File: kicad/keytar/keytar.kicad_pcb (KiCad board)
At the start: 2 copper layers, 70 x 82.5 mm, 32 parts, among them J1 , J2 USB_B, J3 AudioJack2, J4 Conn_01x04, J5 USB_A, J6 Mini-DIN-6-Shielded, J7 Conn_01x04, Q1 BSS138, Q2 BSS138, U1 Pico, U2 MCP73831-2-OT

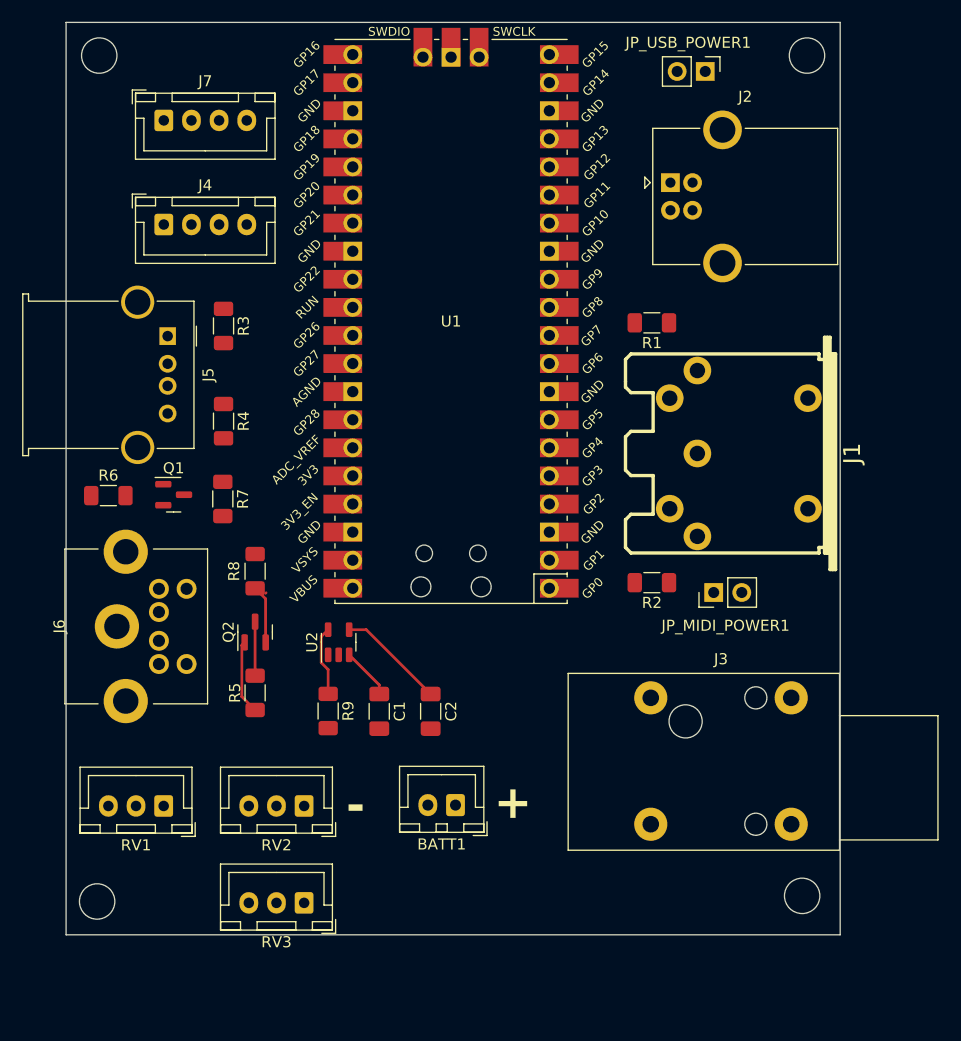
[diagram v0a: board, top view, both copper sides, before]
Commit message: route board
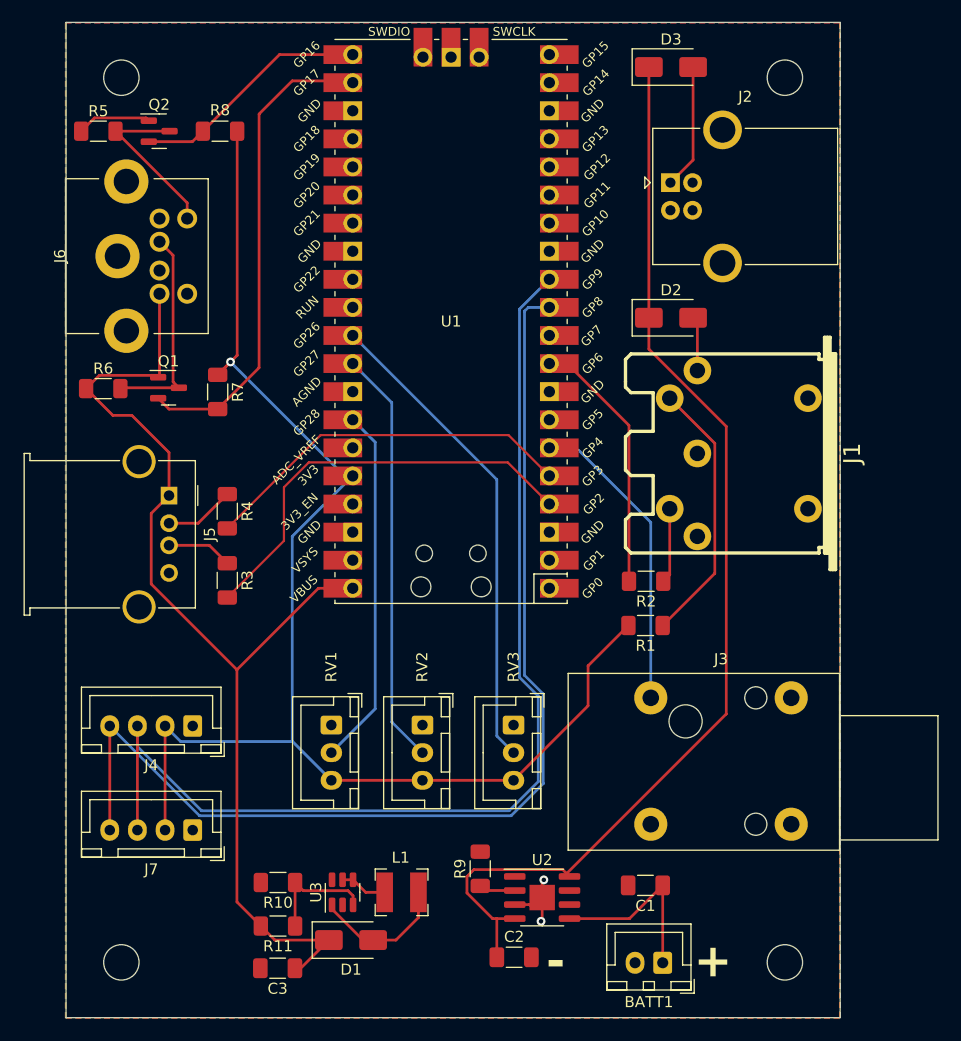
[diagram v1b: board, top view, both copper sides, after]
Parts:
- removed JP_MIDI_POWER1: MIDI Power, Connector_PinHeader_2.54mm:PinHeader_1x02_P2.54mm_Vertical
- removed JP_USB_POWER1: USB Power, Connector_PinHeader_2.54mm:PinHeader_1x02_P2.54mm_Vertical
- added C3: 22u, Capacitor_SMD:C_1206_3216Metric_Pad1.33x1.80mm_HandSolder, F.Cu at (139.1, 140.5)
- added D1: D_Schottky, Diode_SMD:D_SMA, F.Cu at (145.8, 138.0)
- added D2: D_Schottky, Diode_SMD:D_SMA, F.Cu at (174.7, 81.7)
- added D3: D_Schottky, Diode_SMD:D_SMA, F.Cu at (174.7, 59.0)
- added L1: 22u, Inductor_SMD:L_Bourns-SRN4018, F.Cu at (150.3, 133.7)
- added R10: 1k, Resistor_SMD:R_1206_3216Metric_Pad1.30x1.75mm_HandSolder, F.Cu at (139.2, 132.8)
- added R11: 7k5, Resistor_SMD:R_1206_3216Metric_Pad1.30x1.75mm_HandSolder, F.Cu at (139.2, 136.7)
- added U3: MT3608, Package_TO_SOT_SMD:SOT-23-6, F.Cu at (145.0, 133.7)
- C1: value 4u7 -> 22u
- C2: value 4u7 -> 10u
- U2: value MCP73831-2-OT -> ~; footprint Package_TO_SOT_SMD:SOT-23-5 -> Package_SO:HSOP-8-1EP_3.9x4.9mm_P1.27mm_EP2.3x2.3mm
- moved J7 64.2 mm to (131.5, 128.0), turned to 180 degrees
- moved R5 52.7 mm to (122.9, 64.8), turned to 0 degrees
- moved Q2 46.1 mm to (128.4, 64.8), turned to 0 degrees
- moved J4 45.4 mm to (131.5, 118.6), turned to 180 degrees
- moved R8 39.9 mm to (133.9, 64.8), turned to 180 degrees
- moved J6 33.5 mm to (120.0, 76.1)
- moved U2 29.5 mm to (163.1, 134.1), turned to 0 degrees
- moved C1 28.8 mm to (172.4, 133.0), turned to 180 degrees
- moved R1 27.4 mm to (172.4, 109.5)
- moved RV3 24.8 mm to (160.5, 118.5), turned to -90 degrees
- moved BATT1 23.5 mm to (174.0, 140.0)
- moved C2 23.5 mm to (160.5, 139.5), turned to 0 degrees
- moved R3 23.0 mm to (134.6, 105.5)
- moved R9 19.8 mm to (157.5, 131.5), turned to 90 degrees
- moved RV1 16.8 mm to (144.0, 118.5), turned to -90 degrees
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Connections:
- BATT1 pad 1: Net-(BATT1-Pin_1) -> +BATT
- C1 pad 1: Net-(BATT1-Pin_1) -> +BATT
- C2 pad 1: +5V -> VBUS
- J3 pad S: Net-(U1-GPIO22) -> GND
- J3 pad T: GND -> PEDAL
- RV1 pad 1: Net-(U1-AGND) -> GND
- RV1 pad 3: Net-(U1-ADC_VREF) -> +3V3
- RV2 pad 1: Net-(U1-AGND) -> GND
- RV2 pad 3: Net-(U1-ADC_VREF) -> +3V3
- RV3 pad 1: Net-(U1-AGND) -> GND
- RV3 pad 3: Net-(U1-ADC_VREF) -> +3V3
- U1 pad 29: Net-(U1-GPIO22) -> unconnected-(U1-GPIO22-Pad29)
- U1 pad 33: Net-(U1-AGND) -> unconnected-(U1-AGND-Pad33)
- U1 pad 35: Net-(U1-ADC_VREF) -> unconnected-(U1-ADC_VREF-Pad35)
- U1 pad 6: unconnected-(U1-GPIO4-Pad6) -> PEDAL
- U2 pad 1: BAT STATUS -> GND
- U2 pad 2: GND -> Net-(U2-PROG)
- U2 pad 3: Net-(BATT1-Pin_1) -> GND
- U2 pad 4: +5V -> VBUS
- U2 pad 5: Net-(U2-PROG) -> +BATT
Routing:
- net +3V3: track 0.00 -> 127.3 mm, vias 0 -> 1
- net VBUS: track 0.00 -> 102.2 mm
- net Net-(J4-Pin_4): track 0.00 -> 99.0 mm
- net Net-(J4-Pin_3): track 0.00 -> 98.3 mm
- net +5V: track 16.5 -> 102.3 mm
- net Net-(U1-GPIO26_ADC0): track 0.00 -> 43.7 mm
- net PS/2 DATA: track 0.00 -> 43.6 mm
- net USB D+: track 0.00 -> 38.6 mm
- net Net-(U1-GPIO27_ADC1): track 0.00 -> 37.8 mm
- net USB D-: track 0.00 -> 34.1 mm
- net Net-(U1-GPIO28_ADC2): track 0.00 -> 32.6 mm
- net PEDAL: track 0.00 -> 27.8 mm
- net Net-(J1-Pad4): track 0.00 -> 24.2 mm
- net MIDI TX: track 0.00 -> 22.0 mm
- net Net-(Q1-D): track 0.00 -> 19.1 mm
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- added copper zone on B.Cu, net GND
- added copper zone on F.Cu, net GND
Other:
- board size 70 x 82.5 mm -> 70 x 90 mm

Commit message: improve pcb
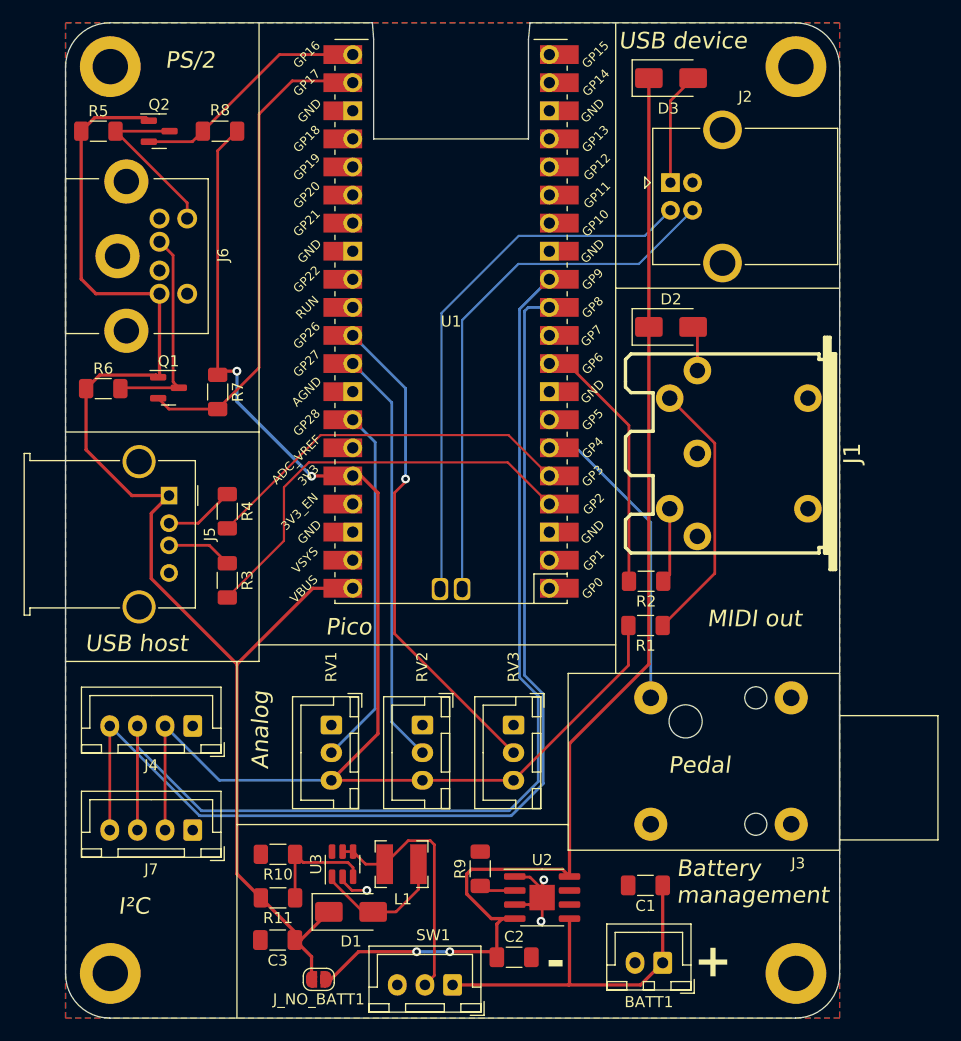
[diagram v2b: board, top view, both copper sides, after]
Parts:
- added J_NO_BATT1: Jumper_2_Open, Jumper:SolderJumper-2_P1.3mm_Open_RoundedPad1.0x1.5mm, F.Cu at (142.9, 141.5)
- added SW1: SW_DPST_x2, Connector_JST:JST_XH_B3B-XH-A_1x03_P2.50mm_Vertical, F.Cu at (155.0, 142.0)
- REF** (x4): value MountingHole_3.2mm_M3 -> MountingHole_3.2mm_M3_ISO14580_Pad; footprint MountingHole:MountingHole_3.2mm_M3 -> MountingHole:MountingHole_3.2mm_M3_ISO14580_Pad
- U1: footprint MCU_RaspberryPi_and_Boards:RPi_Pico_SMD_TH -> keyar-parts:RPi_Pico_debug_hole_USB_SMD_TH
- moved C3 2.55 mm to (139.1, 138.0)
- moved D1 2.55 mm to (145.8, 135.4)
- moved L1 2.55 mm to (150.3, 131.1)
- moved R10 2.55 mm to (139.2, 130.2)
- moved R11 2.55 mm to (139.2, 134.2)
- moved U3 2.55 mm to (145.0, 131.1)
- moved REF** 1.41 mm to (124.0, 141.0)
- moved REF** 1.41 mm to (186.0, 141.0)
- moved REF** 1.41 mm to (124.0, 59.0)
- moved REF** 1.41 mm to (186.0, 59.0)
- moved D3 1.00 mm to (174.7, 60.0)
- moved D2 0.83 mm to (174.7, 82.5)
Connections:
- net Net-(D1-A) renamed /REG_OUT
- net Net-(SW1A-B) renamed /REG_IN
- net USB D+ renamed USB HOST D+
- net USB D- renamed USB HOST D-
- J2 pad 2: unconnected-(J2-D--Pad2) -> USB DEV D-
- J2 pad 3: unconnected-(J2-D+-Pad3) -> USB DEV D+
- J2 pad 5: unconnected-(J2-Shield-Pad5) -> GND
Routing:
- net USB DEV D-: track 0.00 -> 49.6 mm
- net USB DEV D+: track 0.00 -> 49.3 mm
- net +5V: track 102.3 -> 125.1 mm
- net /REG_IN: track 4.28 -> 23.0 mm
- net +BATT: track 16.7 -> 32.9 mm
- net VBUS: track 102.2 -> 113.5 mm, vias 0 -> 2
- net GND: track 5.54 -> 12.2 mm, vias 2 -> 3
- net +3V3: track 127.3 -> 132.6 mm, vias 1 -> 2
- net Net-(D3-A): track 11.3 -> 10.3 mm
- net Net-(U1-GPIO26_ADC0): track 43.7 -> 44.6 mm, vias 0 -> 1
- net Net-(D2-A): track 5.48 -> 4.65 mm
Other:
- outline, holes or cut-outs redrawn
- board text added: "Analog"
- board text added: "Battery management"
- board text added: "I²C"
- board text added: "MIDI out"
- board text added: "PS/2"
- board text added: "Pedal"
- board text added: "Pico"
- board text added: "USB device"
- board text added: "USB host"
